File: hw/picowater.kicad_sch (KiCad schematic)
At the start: 11 parts, among them J1 Conn_01x04_MountingPin, J2 Conn_01x02_MountingPin, J3 Conn_01x06_Pin, J4 UART, U1 Pico

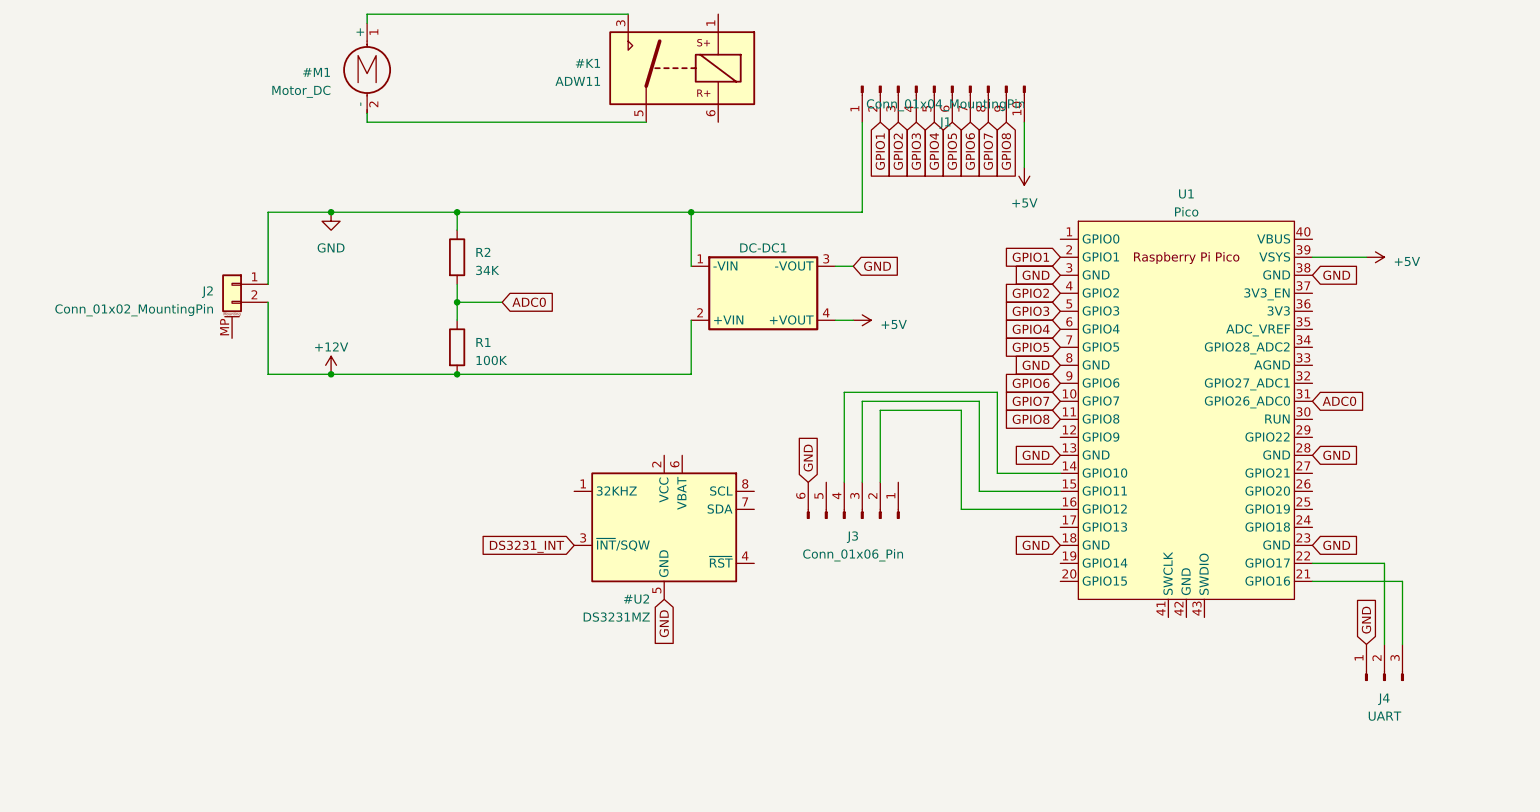
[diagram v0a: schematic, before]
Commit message: update PCB+code
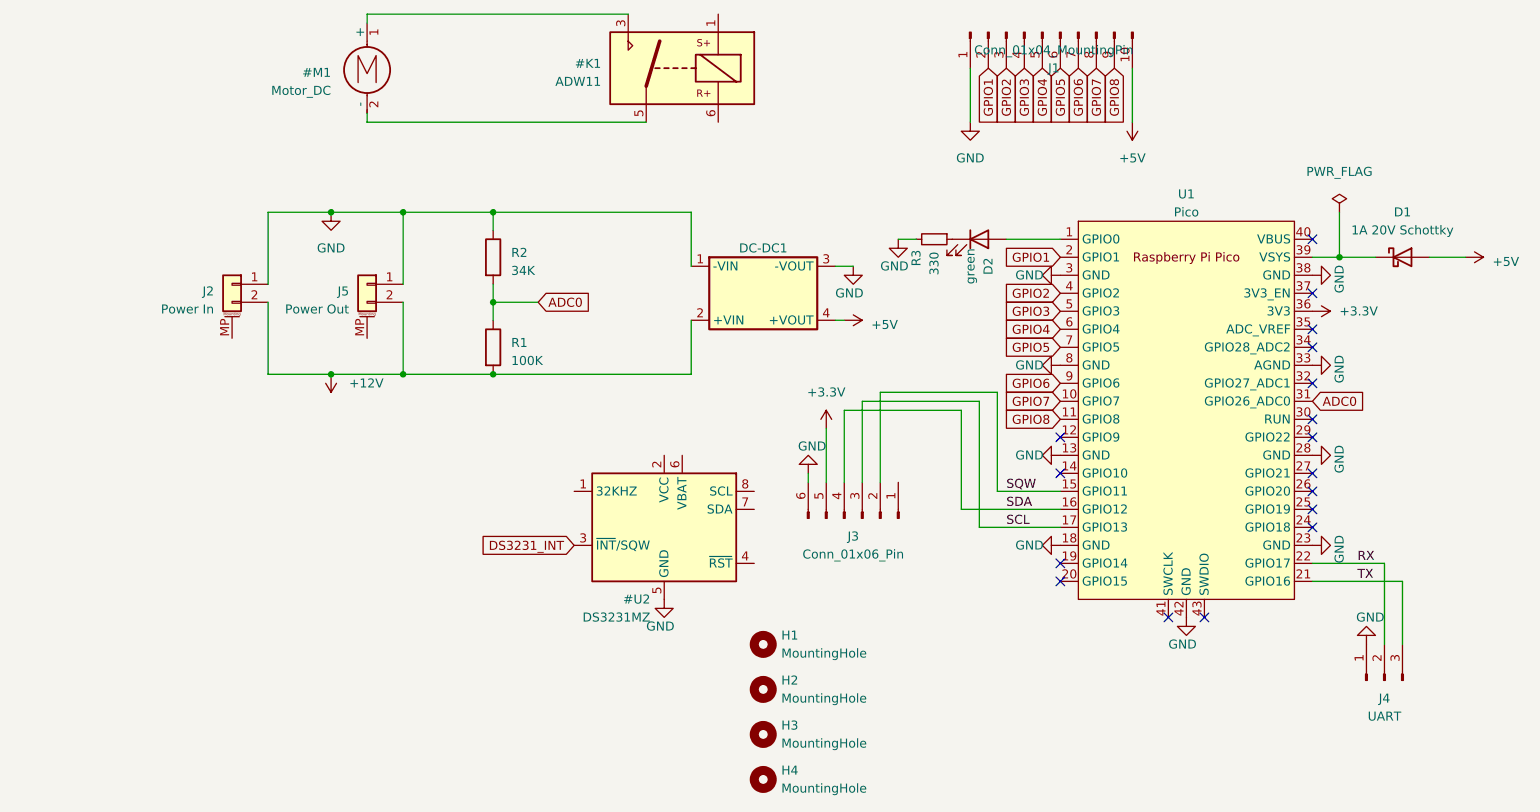
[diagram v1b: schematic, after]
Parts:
- added D1: 1A 20V Schottky, Diode_SMD:D_SOD-123F, symbol Device:D_Schottky
- added D2: green, LED_THT:LED_D3.0mm, symbol Device:LED
- added H1, H2, H3, H4: MountingHole, MountingHole:MountingHole_2.5mm, symbol Mechanical:MountingHole
- added J5: Power Out, Connector_PinHeader_2.54mm:PinHeader_1x02_P2.54mm_Vertical, symbol Connector_Generic_MountingPin:Conn_01x02_MountingPin
- added R3: 330, Resistor_SMD:R_1206_3216Metric_Pad1.30x1.75mm_HandSolder, symbol Device:R_Small
- J2: value Conn_01x02_MountingPin -> Power In
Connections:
- net +12V: now also J5.2 (Pin_2)
- net +5V: now also D1.2 (A); no longer U1.39 (VSYS)
- net GND: now also U1.33 (AGND), U1.42 (GND), J5.1 (Pin_1), R3.2
- net RX: now reaches J4.2 (Pin_2), U1.22 (GPIO17)
- net TX: now reaches J4.3 (Pin_3), U1.21 (GPIO16)
- net at U1.1 (GPIO0): now also D2.2 (A)
- net at U1.14 (GPIO10): no longer J3.4 (Pin_4)
- net SCL: now reaches J3.3 (Pin_3)
- net SCL: now also U1.17 (GPIO13); no longer U1.15 (GPIO11)
- net SDA: now reaches U1.16 (GPIO12)
- net SDA: now also J3.4 (Pin_4); no longer J3.2 (Pin_2)
- net +3.3V: now reaches U1.36 (3V3)
- net +3.3V: now also J3.5 (Pin_5)
- new net: D1.1 (K), U1.39 (VSYS)
- new net: D2.1 (K), R3.1
- new net SQW: J3.2 (Pin_2), U1.15 (GPIO11)
- no-connect marks 0 -> 17
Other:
- moved on the sheet: J1, R1, R2

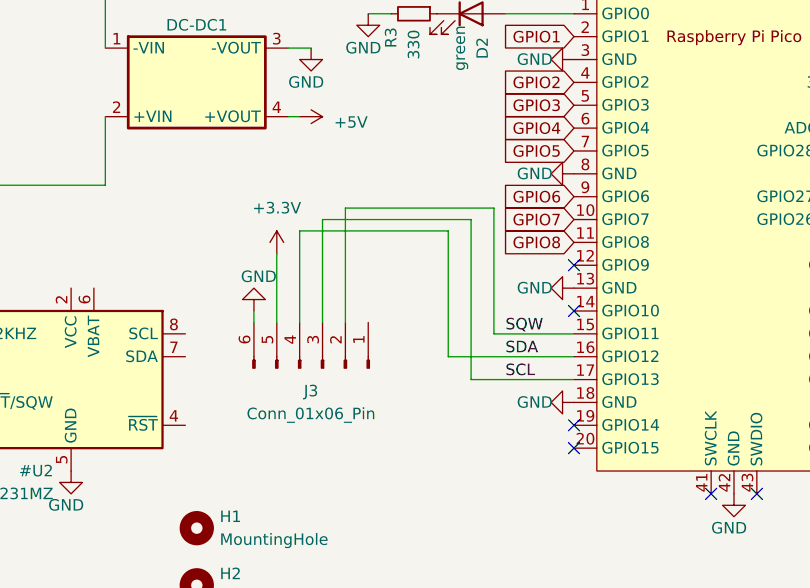
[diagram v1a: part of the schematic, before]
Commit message: pcb update
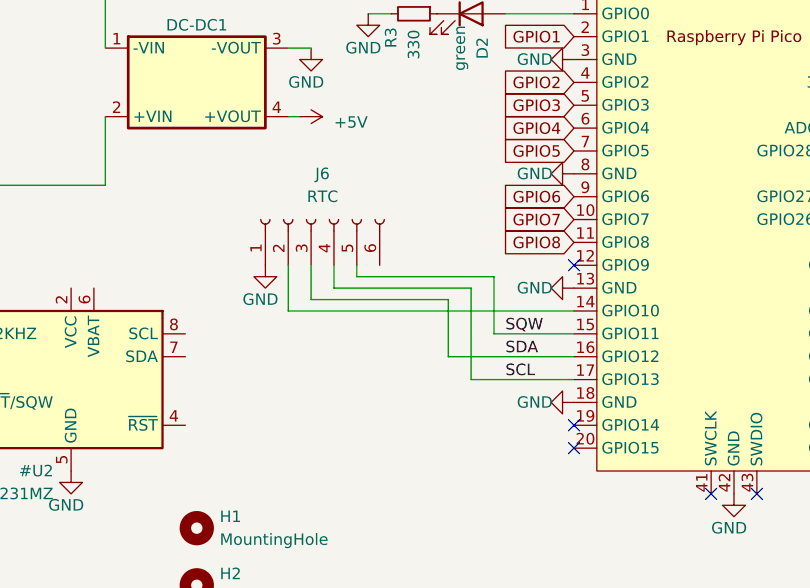
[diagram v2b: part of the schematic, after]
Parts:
- removed J3: Conn_01x06_Pin, Connector_PinSocket_2.54mm:PinSocket_1x06_P2.54mm_Horizontal, symbol Connector:Conn_01x06_Pin
- added J6: RTC, Connector_PinSocket_2.54mm:PinSocket_1x06_P2.54mm_Horizontal, symbol Connector:Conn_01x06_Socket
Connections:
- net GND: now also J6.1 (Pin_1)
- net SCL: now also J6.4 (Pin_4)
- net SDA: now also J6.3 (Pin_3)
- net SQW: now also J6.5 (Pin_5)
- net at U1.14 (GPIO10): now also J6.2 (Pin_2)
- no-connect marks 17 -> 16
